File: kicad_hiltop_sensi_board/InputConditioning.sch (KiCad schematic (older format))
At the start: 50 parts, among them U4 OPA197IDR, U5 OPA197IDR, U6 OPA197IDR, U7 OPA197IDR, U8 OPA197IDR

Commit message: Just about to aad the RTD
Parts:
- C14, C15, C16, C17, C18, C20, C21, C22, C23, C24, C25, C26, C27, C28, C29: symbol device:C -> Sensi_Board-rescue:C-device
- R18, R19, R20, R21, R22, R23, R24, R25, R26, R27, R28, R29, R30, R31, R32, R33, R34, R35, R36, R37, R38, R39, R40, R41, R42, R43, R44, R45, R46, R47: symbol device:R -> Sensi_Board-rescue:R-device
- U4, U5, U6, U7, U8: symbol linear:OPA2340 -> Sensi_Board-rescue:OPA2340-linear
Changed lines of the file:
@@
 EESchema Schematic File Version 4
 LIBS:Sensi_Board-cache
-EELAYER 29 0
+EELAYER 30 0
 EELAYER END
 $Descr A3 11693 16535 portrait
 encoding utf-8
-Sheet 2 8
+Sheet 2 9
 Title ""
 Date ""
@@
 $EndDescr
 $Comp
-L device:R R23
+L Sensi_Board-rescue:R-device R23
 U 1 1 5BB25688
 P 1725 1525
@@
 $EndComp
 $Comp
-L device:R R20
+L Sensi_Board-rescue:R-device R20
 U 1 1 5BB25A8B
 P 1700 2700
@@
 	1550 2700 1400 2700
 $Comp
-L device:C C20
+L Sensi_Board-rescue:C-device C20
 U 1 1 5BB35C7B
 P 4350 1950
@@
 	1425 1525 1575 1525
 $Comp
-L linear:OPA2340 U4
+L Sensi_Board-rescue:OPA2340-linear U4
 U 1 1 5C4E9C83
 P 2800 1625
@@
 $EndComp
 $Comp
-L linear:OPA2340 U4
+L Sensi_Board-rescue:OPA2340-linear U4
 U 2 1 5C4E9E6C
 P 2800 2800
@@
 	3475 3375 3475 2800
 $Comp
-L device:R R30
+L Sensi_Board-rescue:R-device R30
 U 1 1 5C4EF0F1
 P 4050 1625
@@
 	4350 2200 4350 2100
 $Comp
-L device:C C21
+L Sensi_Board-rescue:C-device C21
 U 1 1 5C4F00D3
 P 4350 3125
@@
 $EndComp
 $Comp
-L device:R R31
+L Sensi_Board-rescue:R-device R31
 U 1 1 5C4F00DA
 P 4050 2800
@@
 Connection ~ 4350 2800
 $Comp
-L device:R R24
+L Sensi_Board-rescue:R-device R24
 U 1 1 5C4F2356
 P 1725 3900
@@
 $EndComp
 $Comp
-L device:R R21
+L Sensi_Board-rescue:R-device R21
 U 1 1 5C4F235C
 P 1700 5075
@@
 	1550 5075 1400 5075
 $Comp
-L device:C C22
+L Sensi_Board-rescue:C-device C22
 U 1 1 5C4F2363
 P 4350 4325
@@
 	1425 3900 1575 3900
 $Comp
-L linear:OPA2340 U5
+L Sensi_Board-rescue:OPA2340-linear U5
 U 1 1 5C4F236C
 P 2800 4000
@@
 $EndComp
 $Comp
-L linear:OPA2340 U5
+L Sensi_Board-rescue:OPA2340-linear U5
 U 2 1 5C4F2372
 P 2800 5175
@@
 	3475 5750 3475 5175
 $Comp
-L device:R R32
+L Sensi_Board-rescue:R-device R32
 U 1 1 5C4F2391
 P 4050 4000
@@
 	4350 4575 4350 4475
 $Comp
-L device:C C23
+L Sensi_Board-rescue:C-device C23
 U 1 1 5C4F23A1
 P 4350 5500
@@
 $EndComp
 $Comp
-L device:R R33
+L Sensi_Board-rescue:R-device R33
 U 1 1 5C4F23A7
 P 4050 5175
@@
 Connection ~ 4350 5175
 $Comp
-L device:R R22
+L Sensi_Board-rescue:R-device R22
 U 1 1 5C4F7D07
 P 1700 6350
@@
 $EndComp
 $Comp
-L device:C C24
+L Sensi_Board-rescue:C-device C24
 U 1 1 5C4F7D14
 P 4350 6775
@@
 	1425 6350 1550 6350
 $Comp
-L linear:OPA2340 U6
+L Sensi_Board-rescue:OPA2340-linear U6
 U 1 1 5C4F7D1D
 P 2800 6450
@@
 $EndComp
 $Comp
-L linear:OPA2340 U6
+L Sensi_Board-rescue:OPA2340-linear U6
 U 2 1 5C4F7D23
 P 2975 8575
@@
 	3650 9150 3650 8575
 $Comp
-L device:R R34
+L Sensi_Board-rescue:R-device R34
 U 1 1 5C4F7D42
 P 4050 6450
@@
 	4350 7025 4350 6925
 $Comp
-L device:C C25
+L Sensi_Board-rescue:C-device C25
 U 1 1 5C4F7D52
 P 4525 8900
@@
 $EndComp
 $Comp
-L device:R R35
+L Sensi_Board-rescue:R-device R35
 U 1 1 5C4F7D58
 P 4225 8575
@@
 Connection ~ 4525 8575
 $Comp
-L device:C C14
+L Sensi_Board-rescue:C-device C14
 U 1 1 5C4FA8D8
 P 1925 13225
@@
 $EndComp
 $Comp
-L device:C C15
+L Sensi_Board-rescue:C-device C15
 U 1 1 5C4FABED
 P 2375 13225
@@
 $EndComp
 $Comp
-L device:C C16
+L Sensi_Board-rescue:C-device C16
 U 1 1 5C4FAC61
 P 2825 13225
@@
 $EndComp
 $Comp
-L device:R R18
+L Sensi_Board-rescue:R-device R18
 U 1 1 5C7680D6
 P 1425 8200
@@
 	1425 8475 1425 8350
 $Comp
-L device:R R19
+L Sensi_Board-rescue:R-device R19
 U 1 1 5C76B393
 P 1425 8775
@@
 	1325 7925 1425 7925
 $Comp
-L device:C C26
+L Sensi_Board-rescue:C-device C26
 U 1 1 5C7A1E5F
 P 9950 4175
@@
 $EndComp
 $Comp
-L linear:OPA2340 U7
+L Sensi_Board-rescue:OPA2340-linear U7
 U 1 1 5C7A1E65
 P 8400 3850
@@
 $EndComp
 $Comp
-L linear:OPA2340 U7
+L Sensi_Board-rescue:OPA2340-linear U7
 U 2 1 5C7A1E6B
 P 8400 5600
@@
 	9075 6175 9075 5600
 $Comp
-L device:R R44
+L Sensi_Board-rescue:R-device R44
 U 1 1 5C7A1E84
 P 9650 3850
@@
 	9950 4425 9950 4325
 $Comp
-L device:C C27
+L Sensi_Board-rescue:C-device C27
 U 1 1 5C7A1E94
 P 9950 5925
@@
 $EndComp
 $Comp
-L device:R R45
+L Sensi_Board-rescue:R-device R45
 U 1 1 5C7A1E9A
 P 9650 5600
@@
 $EndComp
 $Comp
-L device:R R36
+L Sensi_Board-rescue:R-device R36
 U 1 1 5C7A1EB5
 P 6850 3475
@@
 	6850 3750 6850 3625
 $Comp
-L device:R R37
+L Sensi_Board-rescue:R-device R37
 U 1 1 5C7A1EBC
 P 6850 4050
@@
 	6225 3200 6850 3200
 $Comp
-L device:R R38
+L Sensi_Board-rescue:R-device R38
 U 1 1 5C7A1ECE
 P 6850 5225
@@
 	6225 4950 6850 4950
 $Comp
-L device:C C28
+L Sensi_Board-rescue:C-device C28
 U 1 1 5C7B0D6B
 P 9975 7800
@@
 $EndComp
 $Comp
-L linear:OPA2340 U8
+L Sensi_Board-rescue:OPA2340-linear U8
 U 1 1 5C7B0D71
 P 8425 7475
@@
 	8325 7100 8325 7175
 $Comp
-L device:R R46
+L Sensi_Board-rescue:R-device R46
 U 1 1 5C7B0D90
 P 9675 7475
@@
 $EndComp
 $Comp
-L device:R R40
+L Sensi_Board-rescue:R-device R40
 U 1 1 5C7B0DC1
 P 6875 7100
@@
 	6250 6825 6875 6825
 $Comp
-L device:C C17
+L Sensi_Board-rescue:C-device C17
 U 1 1 5C809382
 P 3275 13225
@@
 $EndComp
 $Comp
-L device:C C18
+L Sensi_Board-rescue:C-device C18
 U 1 1 5C80943A
 P 3725 13225
@@
 Connection ~ 3275 13475
 $Comp
-L device:R R39
+L Sensi_Board-rescue:R-device R39
 U 1 1 5D36C9C8
 P 6850 5800
@@
 $EndComp
 $Comp
-L device:R R41
+L Sensi_Board-rescue:R-device R41
 U 1 1 5D36CEB4
 P 6875 7675
@@
 $EndComp
 $Comp
-L device:R R43
+L Sensi_Board-rescue:R-device R43
 U 1 1 5D36D0BD
 P 6875 9425
@@
 	6875 9125 6875 9000
 $Comp
-L device:R R42
+L Sensi_Board-rescue:R-device R42
 U 1 1 5C7B0DDA
 P 6875 8850
@@
 	9975 9400 9975 9225
 $Comp
-L device:R R47
+L Sensi_Board-rescue:R-device R47
 U 1 1 5C7B0DA6
 P 9675 9225
@@
 $EndComp
 $Comp
-L device:C C29
+L Sensi_Board-rescue:C-device C29
 U 1 1 5C7B0DA0
 P 9975 9550
@@
 	8725 9225 9100 9225
 $Comp
-L linear:OPA2340 U8
+L Sensi_Board-rescue:OPA2340-linear U8
 U 2 1 5C7B0D77
 P 8425 9225
@@
 Connection ~ 9975 9225
 $Comp
-L device:R R25
+L Sensi_Board-rescue:R-device R25
 U 1 1 5F25C0A4
 P 2000 1775
@@
 	2000 1525 2500 1525
 $Comp
-L device:R R26
+L Sensi_Board-rescue:R-device R26
 U 1 1 5F27EA71
 P 2000 2950
@@
 	2000 3100 2000 3150
 $Comp
-L device:R R27
+L Sensi_Board-rescue:R-device R27
 U 1 1 5F285D99
 P 2000 4200
@@
 	2000 4350 2000 4400
 $Comp
-L device:R R29
+L Sensi_Board-rescue:R-device R29
 U 1 1 5F28D397
 P 2000 6650
@@
 	2000 6800 2000 6850
 $Comp
-L device:R R28
+L Sensi_Board-rescue:R-device R28
 U 1 1 5F294A60
 P 2000 5375

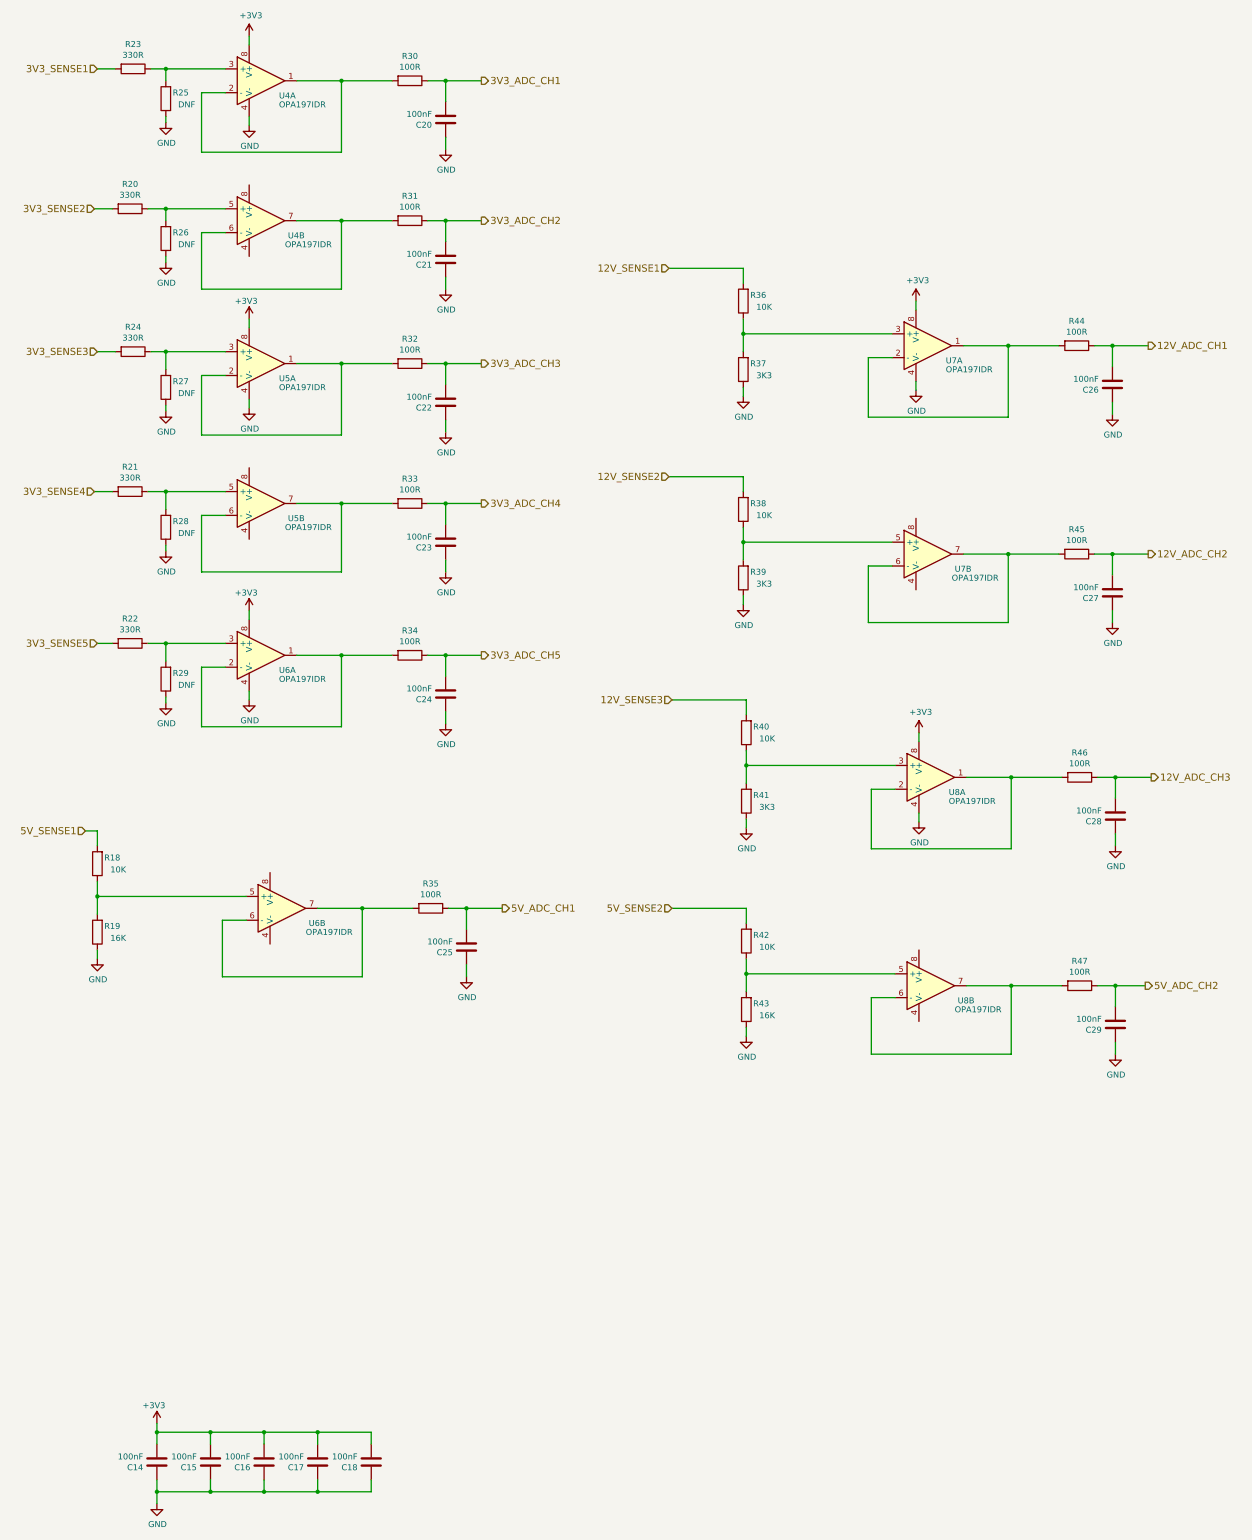
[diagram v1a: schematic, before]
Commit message: updated sensi board for LBBC 04/09/19
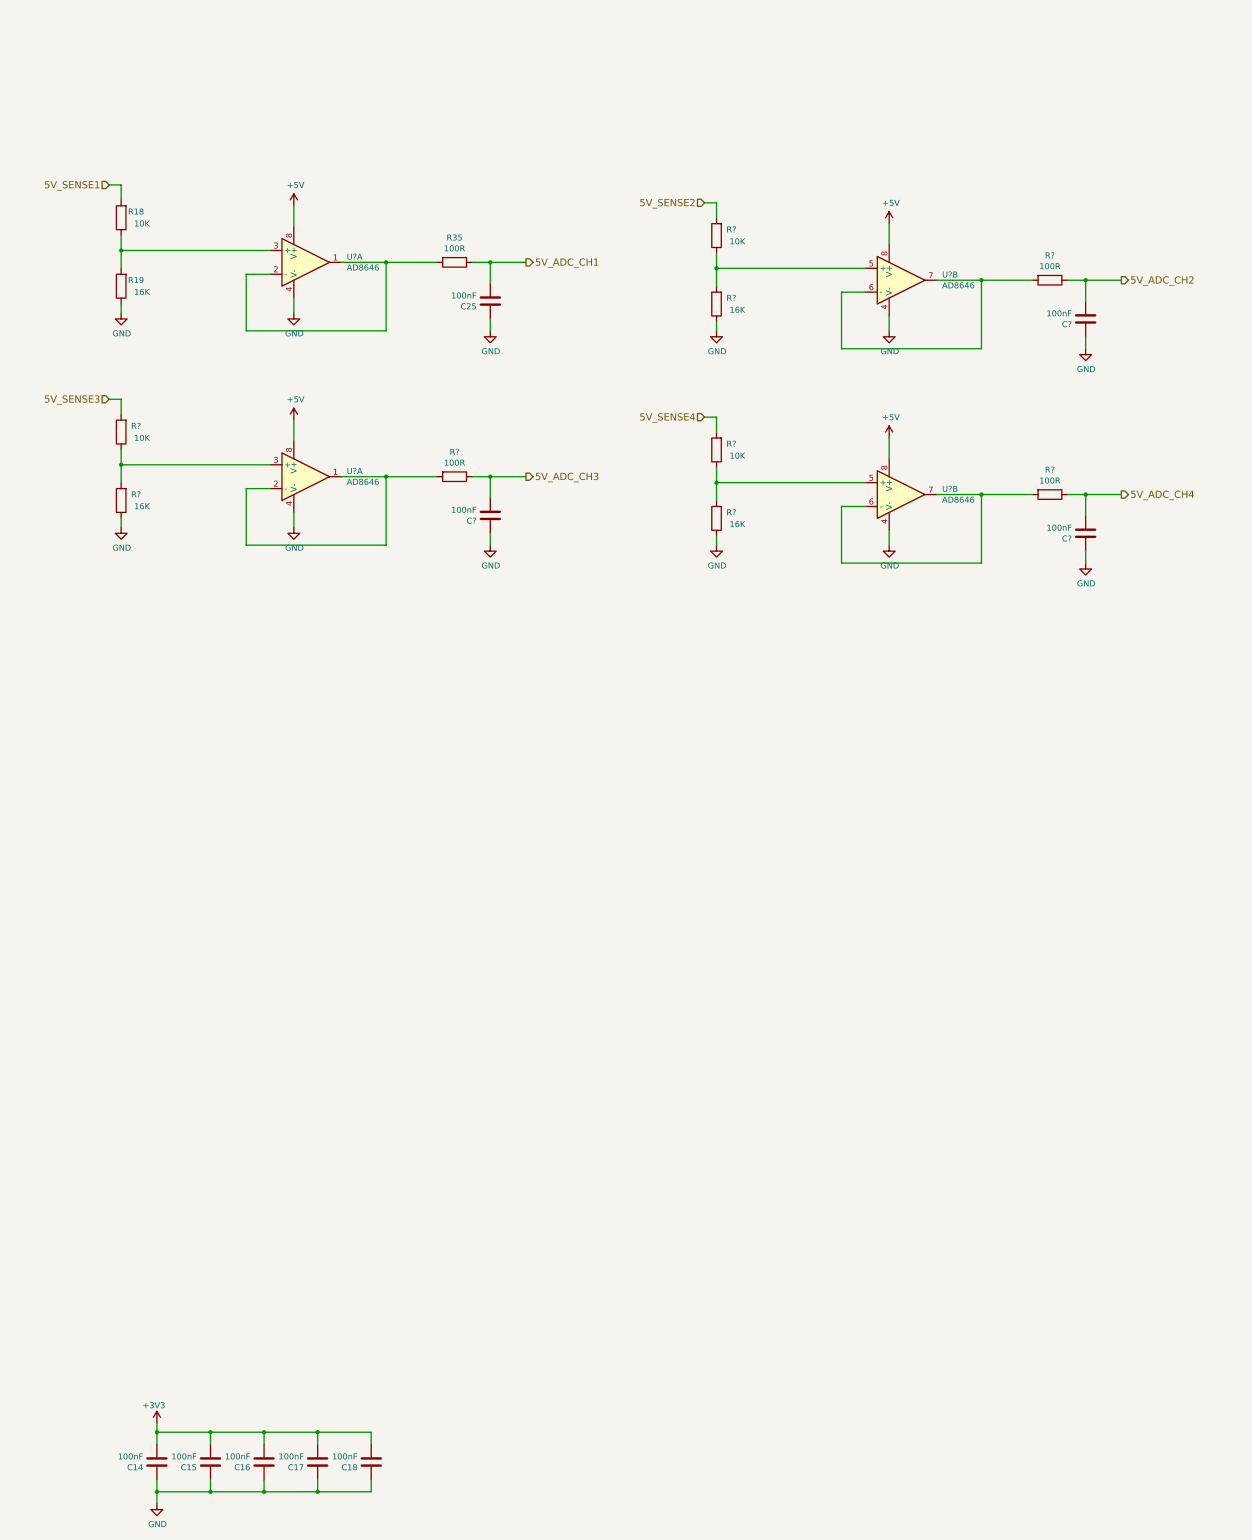
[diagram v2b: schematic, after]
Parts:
- removed C20, C21, C22, C23, C24, C26, C27, C28, C29: 100nF, Capacitor_SMD:C_0603_1608Metric, symbol Sensi_Board-rescue:C-device
- removed R20, R21, R22, R23, R24: 330R, Resistor_SMD:R_0603_1608Metric, symbol Sensi_Board-rescue:R-device
- removed R25, R26, R27, R28, R29: DNF, Resistor_SMD:R_0603_1608Metric, symbol Sensi_Board-rescue:R-device
- removed R30, R31, R32, R33, R34, R44, R45, R46, R47: 100R, Resistor_SMD:R_0603_1608Metric, symbol Sensi_Board-rescue:R-device
- removed R36, R38, R40, R42: 10K, Resistor_SMD:R_0603_1608Metric, symbol Sensi_Board-rescue:R-device
- removed R37, R39, R41: 3K3, Resistor_SMD:R_0603_1608Metric, symbol Sensi_Board-rescue:R-device
- removed R43: 16K, Resistor_SMD:R_0603_1608Metric, symbol Sensi_Board-rescue:R-device
- removed U4, U5, U6, U7, U8: OPA197IDR, Package_SO:SOIC-8_3.9x4.9mm_P1.27mm, symbol Sensi_Board-rescue:OPA2340-linear
- added C? (x3): 100nF, Capacitor_SMD:C_0603_1608Metric, symbol Sensi_Board-rescue:C-device
- added R? (x3): 100R, Resistor_SMD:R_0603_1608Metric, symbol Sensi_Board-rescue:R-device
- added R? (x3): 10K, Resistor_SMD:R_0603_1608Metric, symbol Sensi_Board-rescue:R-device
- added R? (x3): 16K, Resistor_SMD:R_0603_1608Metric, symbol Sensi_Board-rescue:R-device
- added U? (x4): AD8646, symbol Devtank:AD8646
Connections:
- net 5V_ADC_CH2: now also C?.2, R?.1
- net 5V_SENSE2: now also R?.2
- net GND: now also C?.1, C?.1, C?.1, R?.1, R?.1, R?.1, U?.4 (V-), U?.4 (V-), U?.4 (V-), U?.4 (V-)
- net at R18.1, R19.2: now also U?.3 (+)
- net at R35.2: now also U?.1, U?.2 (-)
- new net: R?.1, R?.2, U?.5 (+) (x2)
- new net: R?.2, U?.6 (-), U?.7 (x2)
- new net: R?.2, U?.1, U?.2 (-)
- new net: R?.1, R?.2, U?.3 (+)
- new net +5V: U?.8 (V+), U?.8 (V+), U?.8 (V+), U?.8 (V+)
- new net 5V_ADC_CH3: C?.2, R?.1
- new net 5V_ADC_CH4: C?.2, R?.1
- new net 5V_SENSE3: R?.2
- new net 5V_SENSE4: R?.2
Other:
- moved on the sheet: C25, R18, R19, R35
